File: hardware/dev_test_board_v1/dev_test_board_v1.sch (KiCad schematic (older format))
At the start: 53 parts, among them J1 USB_B_Micro, J2 Conn_SWD, J3 Conn_LCD, J4 Conn_GP, SW1 SW_SPDT, SW2 SW_PUSH, SW3 SW_PUSH, SW4 SW_PUSH, U1 STM32L031C4Tx, U2 FT230XS, U3 LIS2HH12, Y1 8MHz

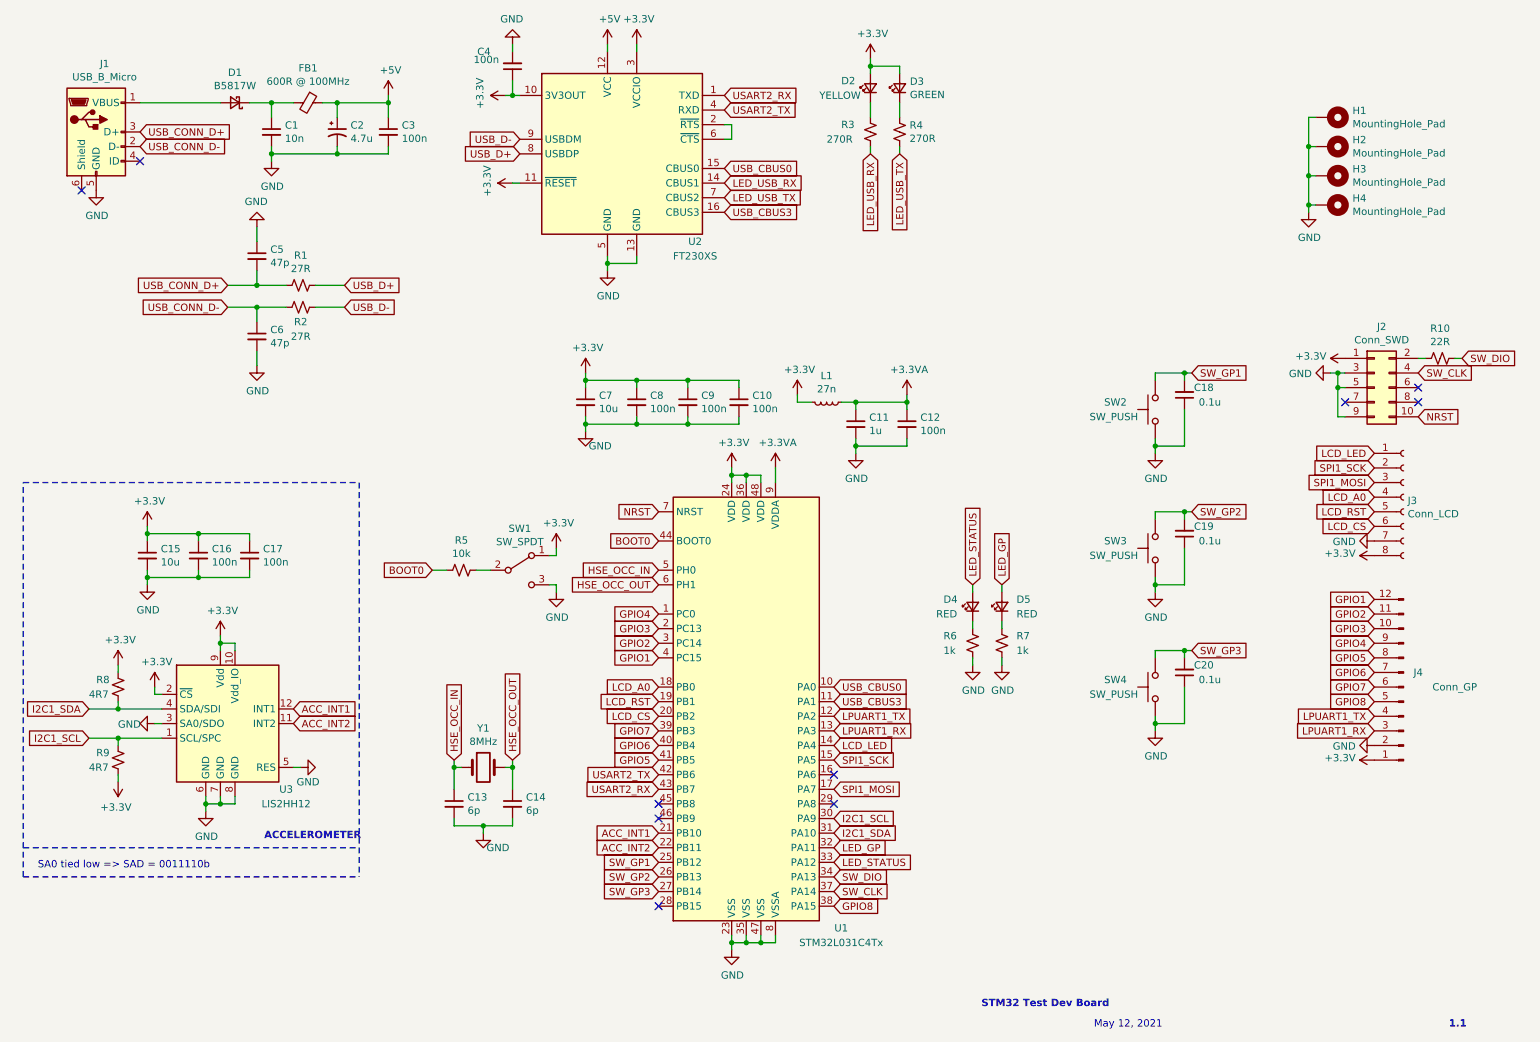
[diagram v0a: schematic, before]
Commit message: Started PCB layout.
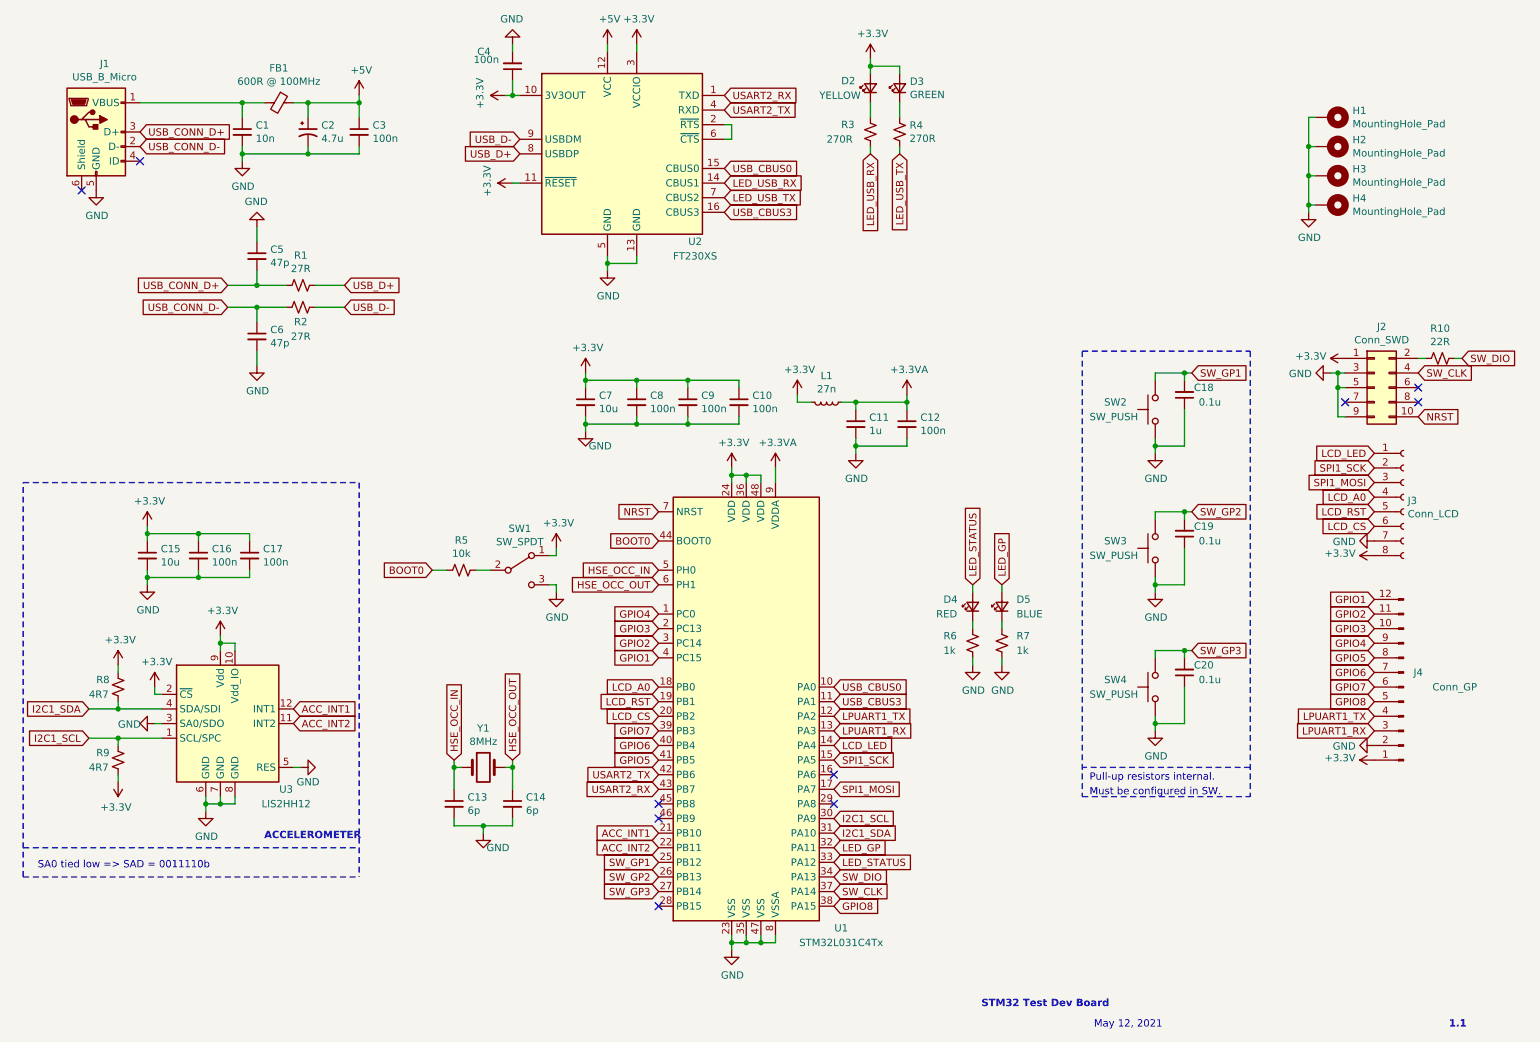
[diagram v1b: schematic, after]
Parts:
- removed D1: B5817W, symbol Device:D_Schottky_Small
- C1, C18, C19, C20, C5, C6: footprint (none) -> Capacitor_SMD:C_0603_1608Metric
- C10, C11, C12, C13, C14, C15, C16, C17, C3, C4, C7, C8, C9: footprint (none) -> Capacitor_SMD:C_0402_1005Metric
- C2: footprint (none) -> Capacitor_SMD:CP_Elec_4x5.4
- D2, D3, D4: footprint (none) -> LED_SMD:LED_0603_1608Metric
- D5: value RED -> BLUE; footprint (none) -> LED_SMD:LED_0603_1608Metric
- FB1: footprint (none) -> Inductor_SMD:L_0805_2012Metric
- H1, H2, H3, H4: footprint (none) -> MountingHole:MountingHole_2.7mm_M2.5_Pad_Via
- J1: footprint (none) -> Connector_USB:USB_Micro-B_GCT_USB3076-30-A
- J2: footprint (none) -> Connector_PinHeader_1.27mm:PinHeader_2x05_P1.27mm_Vertical
- J3: footprint (none) -> Connector_PinSocket_2.54mm:PinSocket_1x08_P2.54mm_Vertical
- J4: footprint (none) -> Connector_PinHeader_2.54mm:PinHeader_1x12_P2.54mm_Vertical
- L1: footprint (none) -> Inductor_SMD:L_0603_1608Metric
- R1, R10, R2, R5, R8, R9: footprint (none) -> Resistor_SMD:R_0402_1005Metric
- R3, R4, R6, R7: footprint (none) -> Resistor_SMD:R_0603_1608Metric
- SW1: footprint (none) -> Button_Switch_SMD:SW_SPDT_PCM12
- SW2, SW3, SW4: footprint (none) -> Button_Switch_SMD:SW_Push_1P1T_NO_6x6mm_H9.5mm
- Y1: footprint (none) -> tyjba_footprints:Crystal_NX8045GB
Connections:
- net at J1.1 (VBUS): now also C1.1, FB1.2
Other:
- note added: "Must be configured in SW."
- note added: "Pull-up resistors internal.\n"
- moved on the sheet: C1, C2, C3, FB1

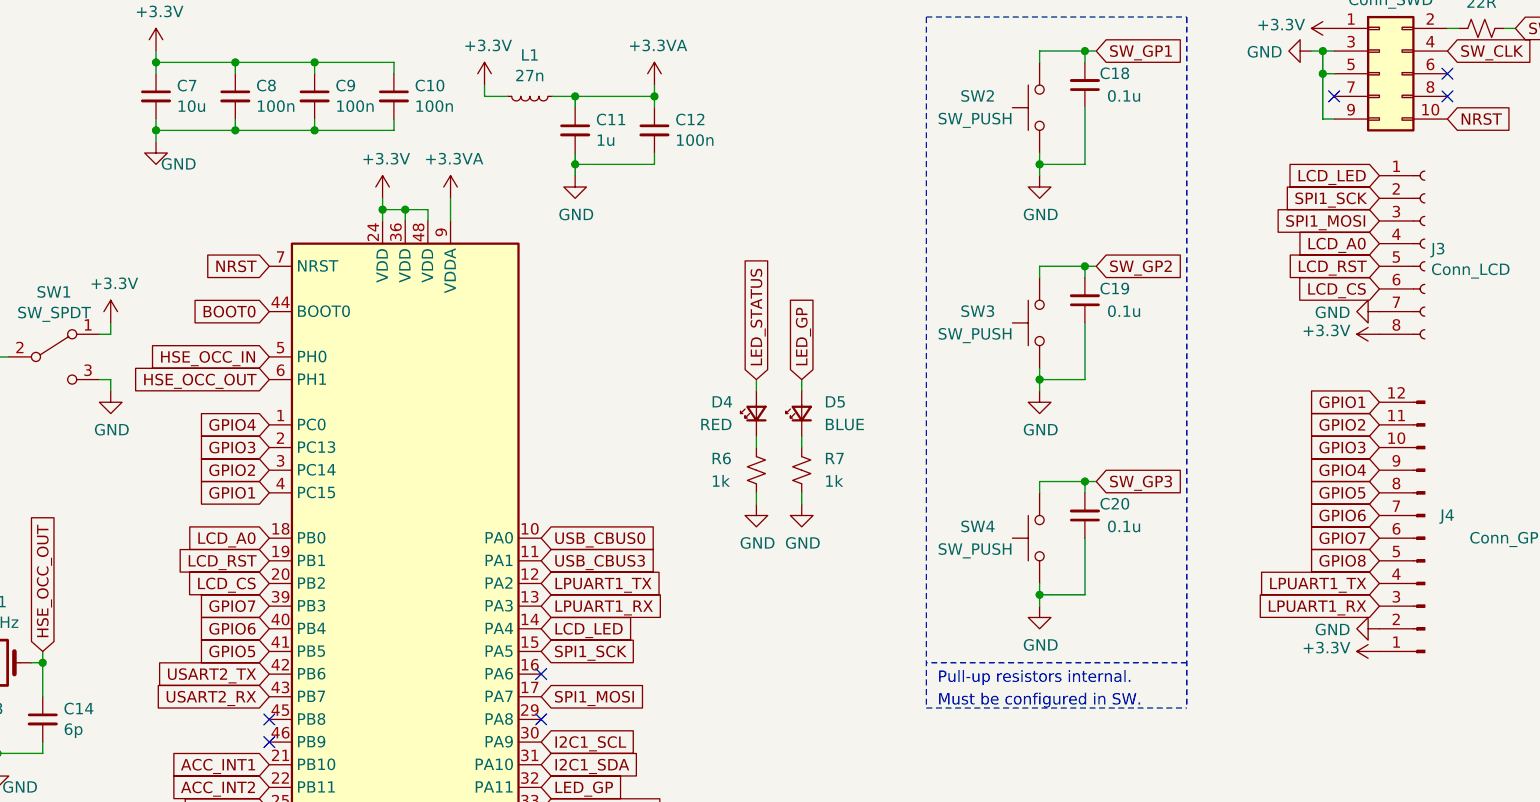
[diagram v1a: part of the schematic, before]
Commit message: Draft layout complete.
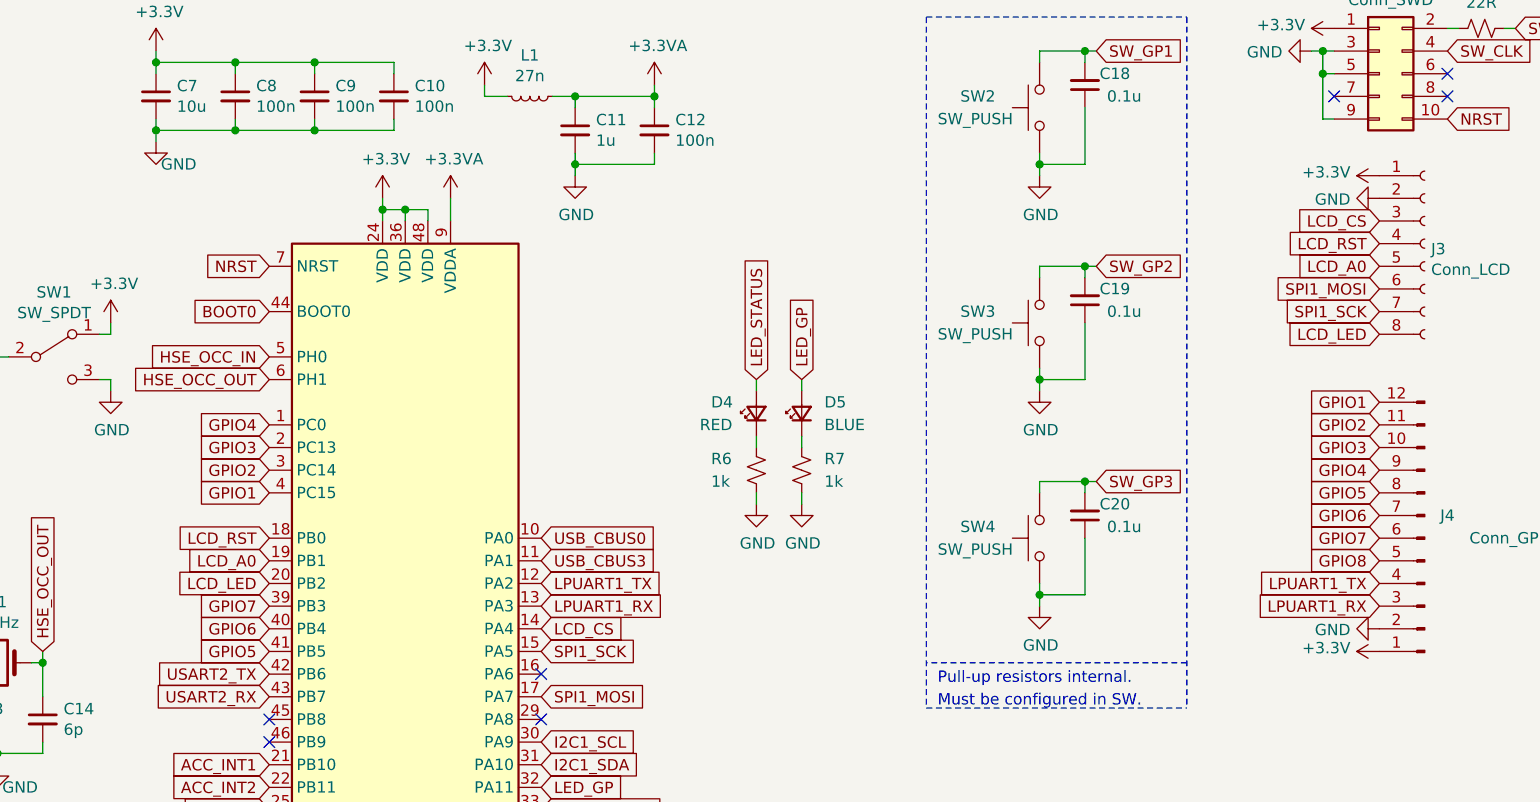
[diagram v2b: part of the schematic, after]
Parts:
- SW1: footprint Button_Switch_SMD:SW_SPDT_PCM12 -> tyjba_footprints:SW_Unknown_SPDT_Straight
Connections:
- net +3V3: now also J3.1 (Pin_1); no longer J3.8 (Pin_8)
- net GND: now also J3.2 (Pin_2); no longer J3.7 (Pin_7)
- net LCD_A0: now also J3.5 (Pin_5), U1.19 (PB1); no longer J3.4 (Pin_4), U1.18 (PB0)
- net LCD_CS: now also J3.3 (Pin_3), U1.14 (PA4); no longer J3.6 (Pin_6), U1.20 (PB2)
- net LCD_LED: now also J3.8 (Pin_8), U1.20 (PB2); no longer J3.1 (Pin_1), U1.14 (PA4)
- net LCD_RST: now also J3.4 (Pin_4), U1.18 (PB0); no longer J3.5 (Pin_5), U1.19 (PB1)
- net SPI1_MOSI: now also J3.6 (Pin_6); no longer J3.3 (Pin_3)
- net SPI1_SCK: now also J3.7 (Pin_7); no longer J3.2 (Pin_2)
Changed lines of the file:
@@
 L power:GND #PWR0125
 U 1 1 609DBE90
-P 10050 4300
-F 0 "#PWR0125" H 10050 4050 50  0001 C CNN
-F 1 "GND" V 10055 4172 50  0000 R CNN
-F 2 "" H 10050 4300 50  0001 C CNN
-F 3 "" H 10050 4300 50  0001 C CNN
-	1    10050 4300
+P 10050 3800
+F 0 "#PWR0125" H 10050 3550 50  0001 C CNN
+F 1 "GND" V 10055 3672 50  0000 R CNN
+F 2 "" H 10050 3800 50  0001 C CNN
+F 3 "" H 10050 3800 50  0001 C CNN
+	1    10050 3800
 	0    1    1    0
 $EndComp
@@
 L power:+3.3V #PWR0124
 U 1 1 609DA543
-P 10050 4400
-F 0 "#PWR0124" H 10050 4250 50  0001 C CNN
-F 1 "+3.3V" V 10065 4528 50  0000 L CNN
-F 2 "" H 10050 4400 50  0001 C CNN
-F 3 "" H 10050 4400 50  0001 C CNN
-	1    10050 4400
+P 10050 3700
+F 0 "#PWR0124" H 10050 3550 50  0001 C CNN
+F 1 "+3.3V" V 10065 3828 50  0000 L CNN
+F 2 "" H 10050 3700 50  0001 C CNN
+F 3 "" H 10050 3700 50  0001 C CNN
+	1    10050 3700
 	0    -1   -1   0
 $EndComp
+Text GLabel 10050 4200 0    50   Input ~ 0
+SPI1_MOSI
+Text GLabel 10050 4300 0    50   Input ~ 0
+SPI1_SCK
 Text GLabel 10050 3900 0    50   Input ~ 0
-SPI1_MOSI
-Text GLabel 10050 3800 0    50   Input ~ 0
-SPI1_SCK
-Text GLabel 10050 4200 0    50   Input ~ 0
 LCD_CS
+Text GLabel 10050 4000 0    50   Input ~ 0
+LCD_RST
 Text GLabel 10050 4100 0    50   Input ~ 0
-LCD_RST
-Text GLabel 10050 4000 0    50   Input ~ 0
 LCD_A0
-Text GLabel 10050 3700 0    50   Input ~ 0
+Text GLabel 10050 4400 0    50   Input ~ 0
 LCD_LED
 $Comp
@@
 Text GLabel 6350 6500 2    50   Input ~ 0
 LED_STATUS
+Text GLabel 6350 5700 2    50   Input ~ 0
+LCD_CS
+Text GLabel 5150 5300 0    50   Input ~ 0
+LCD_RST
+Text GLabel 5150 5400 0    50   Input ~ 0
+LCD_A0
 Text GLabel 5150 5500 0    50   Input ~ 0
-LCD_CS
-Text GLabel 5150 5400 0    50   Input ~ 0
-LCD_RST
-Text GLabel 5150 5300 0    50   Input ~ 0
-LCD_A0
-Text GLabel 6350 5700 2    50   Input ~ 0
 LCD_LED
 Text GLabel 6350 5400 2    50   Input ~ 0
@@
 F 0 "SW1" H 4200 4785 50  0000 C CNN
 F 1 "SW_SPDT" H 4200 4694 50  0000 C CNN
-F 2 "Button_Switch_SMD:SW_SPDT_PCM12" H 4200 4500 50  0001 C CNN
+F 2 "tyjba_footprints:SW_Unknown_SPDT_Straight" H 4200 4500 50  0001 C CNN
 F 3 "~" H 4200 4500 50  0001 C CNN
 	1    4200 4500
